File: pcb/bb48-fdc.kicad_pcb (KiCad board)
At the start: 2 copper layers, 83.8 x 50.1 mm, 10 parts, among them J1 FDD 34-pin host, U1 74LS06, U2 74LS06, U3 74LVC14

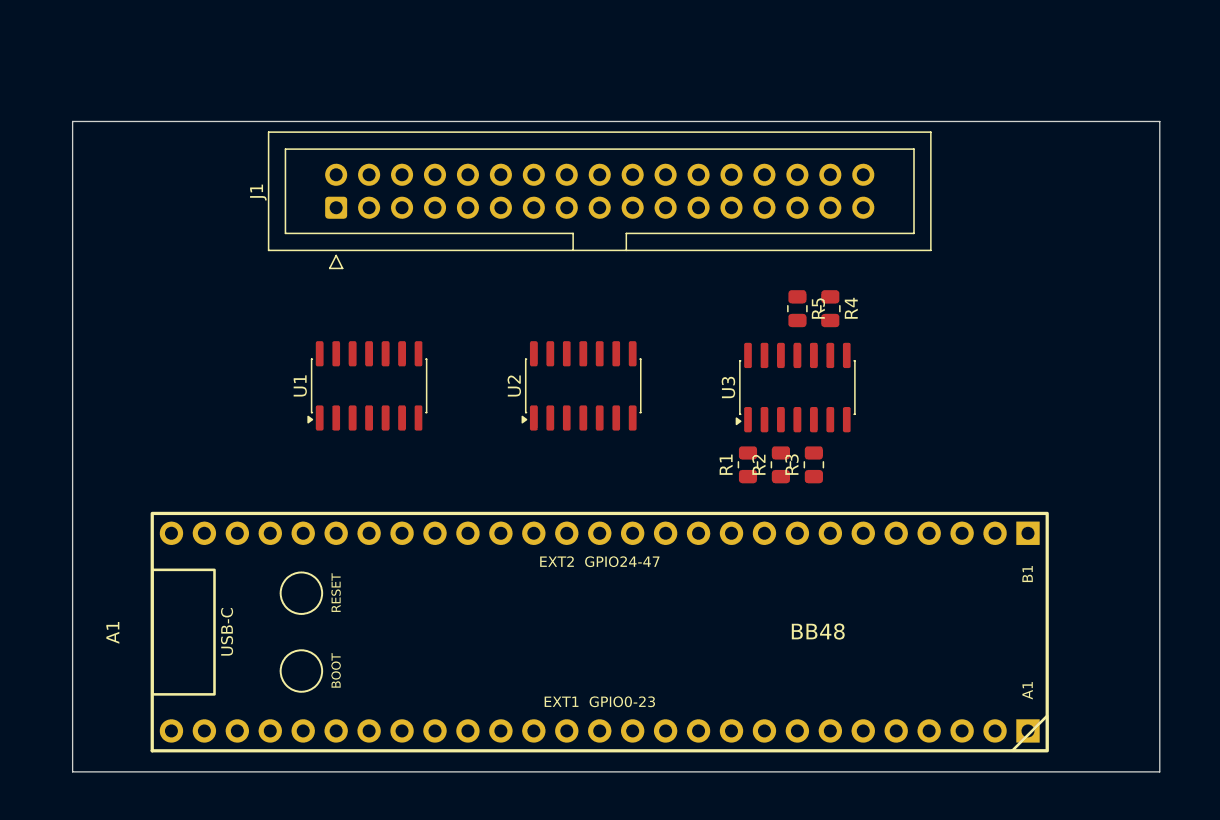
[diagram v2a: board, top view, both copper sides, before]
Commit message: Initial design PCB
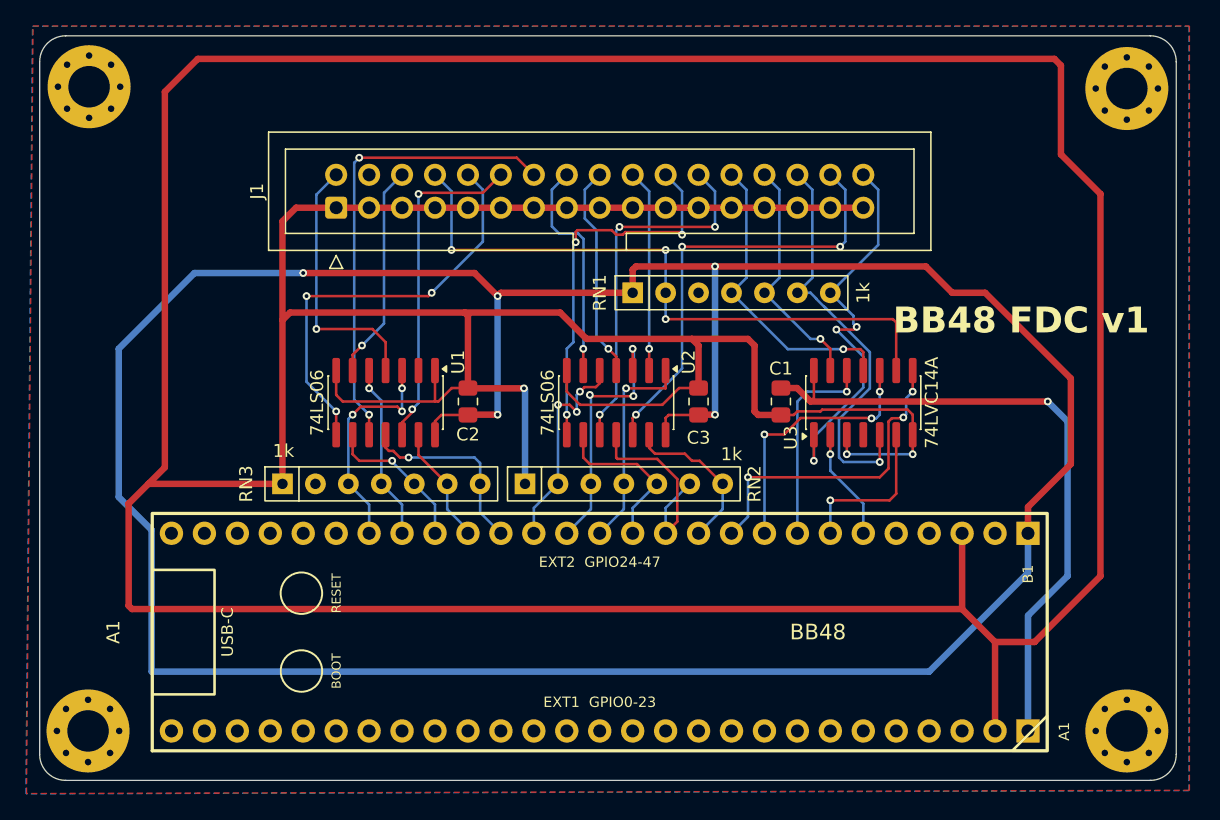
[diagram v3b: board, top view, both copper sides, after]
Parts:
- removed R1, R2, R3, R4, R5: 1k, Resistor_SMD:R_0805_2012Metric
- added C1: 0.1uF, Capacitor_SMD:C_0805_2012Metric_Pad1.18x1.45mm_HandSolder, F.Cu at (74.9, 47.0)
- added C2: 0.1uF, Capacitor_SMD:C_0805_2012Metric_Pad1.18x1.45mm_HandSolder, F.Cu at (50.8, 47.0)
- added C3: 0.1uF, Capacitor_SMD:C_0805_2012Metric_Pad1.18x1.45mm_HandSolder, F.Cu at (68.6, 47.0)
- added H1: MountingHole, MountingHole:MountingHole_3.2mm_M3_Pad_Via, F.Cu at (21.5, 72.4)
- added H2: MountingHole, MountingHole:MountingHole_3.2mm_M3_Pad_Via, F.Cu at (21.6, 22.7)
- added H3: MountingHole, MountingHole:MountingHole_3.2mm_M3_Pad_Via, F.Cu at (101.6, 72.4)
- added H4: MountingHole, MountingHole:MountingHole_3.2mm_M3_Pad_Via, F.Cu at (101.6, 22.9)
- added RN1: 1k, Resistor_THT:R_Array_SIP7, F.Cu at (63.5, 38.6)
- added RN2: 1k, Resistor_THT:R_Array_SIP7, F.Cu at (55.2, 53.3)
- added RN3: 1k, Resistor_THT:R_Array_SIP7, F.Cu at (36.5, 53.3)
- U3: value 74LVC14 -> 74LVC14A
- moved U3 5.21 mm to (81.3, 47.1)
- moved U2 2.85 mm to (62.2, 47.1), turned to -90 degrees
- moved U1 1.81 mm to (44.5, 47.1), turned to -90 degrees
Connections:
- net FDC_DRVSA renamed FDC_DRIVE_A_DS2
- net FDC_RDATA renamed FDC_READ_DATA
- net ~{FDD_DRVSA} renamed ~{FDD_DRIVE_A} / ~{FDD_DS2}
- A1 pad B11: FDC_SIDE1 -> FDC_SIDE_1
- A1 pad B12: FDC_WGATE -> FDC_WRITE_GATE
- A1 pad B13: FDC_WDATA -> FDC_WRITE_DATA
- A1 pad B15: FDC_DIR -> FDC_DIRECTION
- A1 pad B16: FDC_MOTEB -> FDC_MOTOR_B_MOTOR_ON
- A1 pad B18: FDC_DRVSB -> FDC_DRIVE_B_DS1
- A1 pad B19: FDC_MOTEA -> FDC_MOTOR_A_DS0
- A1 pad B20: FDC_DENSEL -> FDC_DS3
- A1 pad B21: unconnected-(A1-GPIO41/ADC1-PadB21) -> FDC_DENSITY_SELECT
- A1 pad B6: FDC_DSKCHG -> FDC_DISK_CHANGE_READY
- A1 pad B8: FDC_WPT -> FDC_WRITE_PROTECT
- A1 pad B9: FDC_TRK0 -> FDC_TRACK_0
- J1 pad 10: ~{FDD_MOTEA} -> ~{FDD_MOTOR_A} / ~{FDD_DS0}
- J1 pad 12: ~{FDD_DRVSB} -> ~{FDD_DRIVE_B} / ~{FDD_DS1}
- J1 pad 16: ~{FDD_MOTEB} -> ~{FDD_MOTOR_B} / ~{FDD_MOTOR_ON}
- J1 pad 18: ~{FDD_DIR} -> ~{FDD_DIRECTION}
- J1 pad 2: ~{FDD_DENSEL} -> ~{FDD_DENSITY_SELECT} / ~{FDD_DISK_CHANGE} / NC
- J1 pad 22: ~{FDD_WDATA} -> ~{FDD_WRITE_DATA}
- J1 pad 24: ~{FDD_WGATE} -> ~{FDD_WRITE_GATE}
- J1 pad 26: ~{FDD_TRK0} -> ~{FDD_TRACK_0}
- J1 pad 28: ~{FDD_WPT} -> ~{FDD_WRITE_PROTECT}
- J1 pad 30: ~{FDD_RDATA} -> ~{FDD_READ_DATA}
- J1 pad 32: ~{FDD_SIDE1} -> ~{FDD_SIDE_1}
- J1 pad 34: ~{FDD_DSKCHG} -> ~{FDD_DISK_CHANGE} / ~{FDD_READY}
- J1 pad 6: unconnected-(J1-NC-Pad6) -> ~{FDD_DS3} / NC
- U1 pad 1: FDC_DENSEL -> GND
- U1 pad 12: ~{FDD_MOTEA} -> ~{FDD_DRIVE_B} / ~{FDD_DS1}
- U1 pad 13: FDC_MOTEA -> FDC_DRIVE_B_DS1
- U1 pad 2: ~{FDD_DENSEL} -> unconnected-(U1-Pad2)
- U1 pad 3: FDC_DRVSB -> FDC_DENSITY_SELECT
- U1 pad 4: ~{FDD_DRVSB} -> ~{FDD_DENSITY_SELECT} / ~{FDD_DISK_CHANGE} / NC
- U1 pad 5: FDC_MOTEB -> FDC_DS3
- U1 pad 6: ~{FDD_MOTEB} -> ~{FDD_DS3} / NC
- U1 pad 8: ~{FDD_DIR} -> ~{FDD_MOTOR_A} / ~{FDD_DS0}
- U1 pad 9: FDC_DIR -> FDC_MOTOR_A_DS0
- U2 pad 10: unconnected-(U2-Pad10) -> ~{FDD_WRITE_GATE}
- U2 pad 11: GND -> FDC_WRITE_GATE
- U2 pad 12: unconnected-(U2-Pad12) -> ~{FDD_SIDE_1}
- U2 pad 13: GND -> FDC_SIDE_1
- U2 pad 3: FDC_WDATA -> FDC_DIRECTION
- U2 pad 4: ~{FDD_WDATA} -> ~{FDD_DIRECTION}
- U2 pad 5: FDC_WGATE -> FDC_MOTOR_B_MOTOR_ON
- U2 pad 6: ~{FDD_WGATE} -> ~{FDD_MOTOR_B} / ~{FDD_MOTOR_ON}
- U2 pad 8: ~{FDD_SIDE1} -> ~{FDD_WRITE_DATA}
- U2 pad 9: FDC_SIDE1 -> FDC_WRITE_DATA
- U3 pad 1: Net-(R1-Pad2) -> ~{FDD_DISK_CHANGE} / ~{FDD_READY}
- U3 pad 10: FDC_WPT -> FDC_TRACK_0
- U3 pad 11: Net-(R5-Pad2) -> ~{FDD_TRACK_0}
- U3 pad 12: unconnected-(U3-Pad12) -> FDC_WRITE_PROTECT
- U3 pad 13: GND -> ~{FDD_WRITE_PROTECT}
- U3 pad 2: FDC_INDEX -> FDC_DISK_CHANGE_READY
- U3 pad 3: Net-(R2-Pad2) -> GND
- U3 pad 4: FDC_TRK0 -> unconnected-(U3-Pad4)
- U3 pad 5: Net-(R3-Pad2) -> ~{FDD_READ_DATA}
- U3 pad 8: FDC_DSKCHG -> FDC_INDEX
- U3 pad 9: Net-(R4-Pad2) -> ~{FDD_INDEX}
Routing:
- net GND: track 0.00 -> 432.9 mm, vias 0 -> 3
- net +5V: track 0.00 -> 227.0 mm, vias 0 -> 5
- net +3V3: track 0.00 -> 50.8 mm, vias 0 -> 1
- net ~{FDD_INDEX}: track 0.00 -> 49.8 mm, vias 0 -> 3
- net ~{FDD_DRIVE_A} / ~{FDD_DS2}: track 0.00 -> 36.0 mm, vias 0 -> 2
- net ~{FDD_SIDE_1}: track 0.00 -> 34.5 mm, vias 0 -> 3
- net ~{FDD_MOTOR_A} / ~{FDD_DS0}: track 0.00 -> 32.6 mm, vias 0 -> 3
- net ~{FDD_READ_DATA}: track 0.00 -> 32.0 mm, vias 0 -> 1
- net ~{FDD_DISK_CHANGE} / ~{FDD_READY}: track 0.00 -> 30.8 mm, vias 0 -> 3
- net ~{FDD_WRITE_DATA}: track 0.00 -> 29.6 mm, vias 0 -> 3
- net ~{FDD_WRITE_GATE}: track 0.00 -> 28.6 mm, vias 0 -> 3
- net ~{FDD_DRIVE_B} / ~{FDD_DS1}: track 0.00 -> 26.1 mm, vias 0 -> 2
- net FDC_INDEX: track 0.00 -> 24.8 mm, vias 0 -> 3
- net ~{FDD_TRACK_0}: track 0.00 -> 23.5 mm, vias 0 -> 1
- net FDC_TRACK_0: track 0.00 -> 20.6 mm, vias 0 -> 3
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- added copper zone on B.Cu, net +5V
- added copper zone on F.Cu, net GND
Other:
- board size 83.8 x 50.1 mm -> 87.6 x 57.4 mm
- board text added: "BB48 FDC v1"
